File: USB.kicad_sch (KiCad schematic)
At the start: 13 parts, among them J2 USB_B_Micro, U6 FT230XS, U7 USBLC6-2SC6

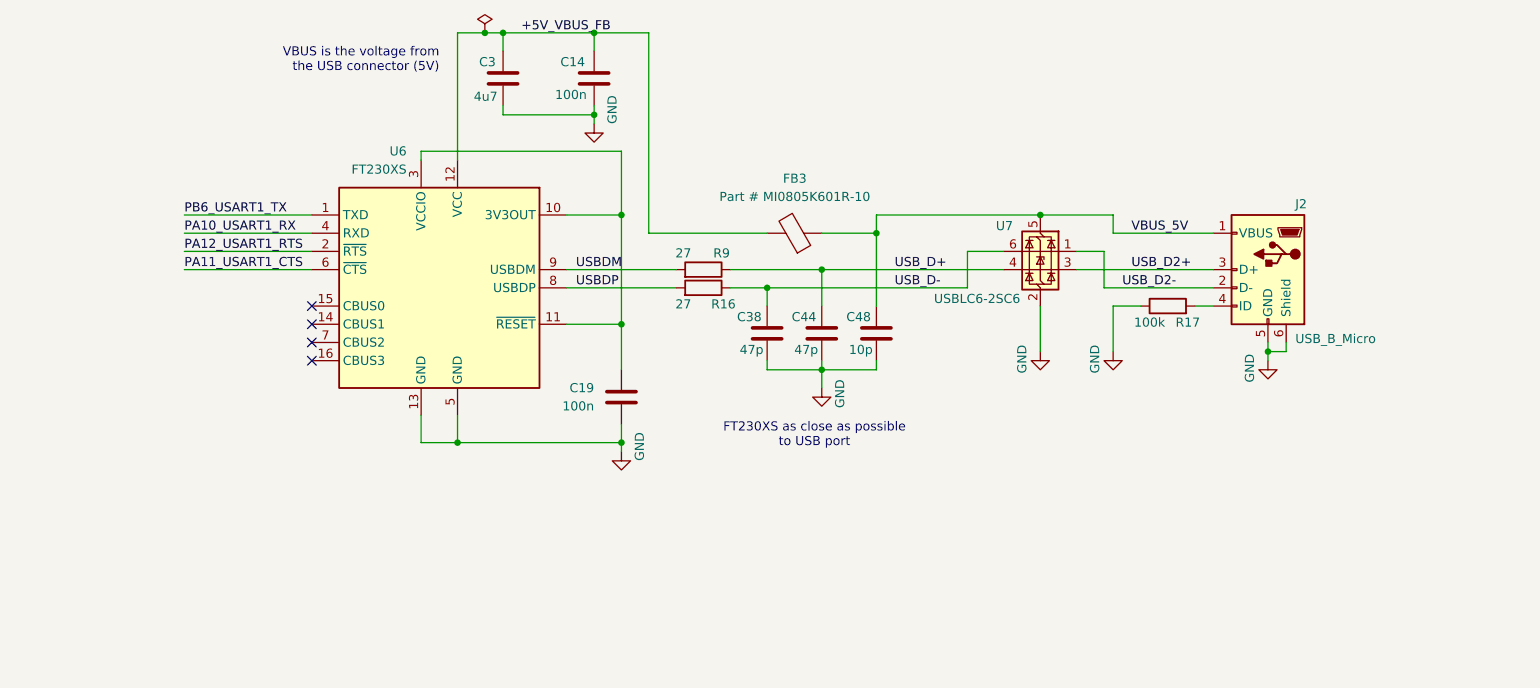
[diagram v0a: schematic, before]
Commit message: Update
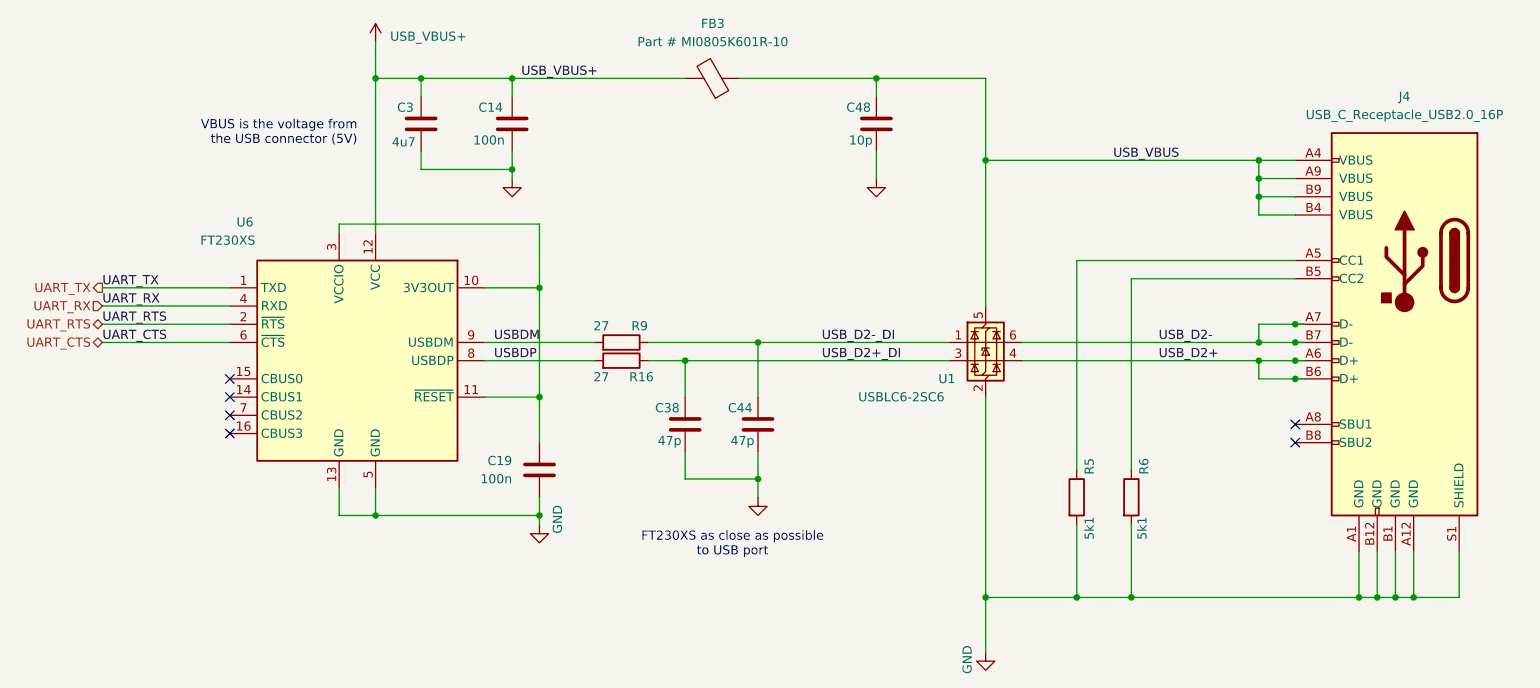
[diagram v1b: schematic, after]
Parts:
- removed J2: USB_B_Micro, Connector_USB:USB_Micro-B_XKB_U254-051T-4BH83-F1S, symbol Connector:USB_B_Micro
- removed R17: 100k, Resistor_SMD:R_0805_2012Metric, symbol Device:R
- removed U7: USBLC6-2SC6, Package_TO_SOT_SMD:SOT-23-6, symbol Power_Protection:USBLC6-2SC6
- added J4: USB_C_Receptacle_USB2.0_16P, Connector_USB:USB_C_Receptacle_HRO_TYPE-C-31-M-12, symbol Connector:USB_C_Receptacle_USB2.0_16P
- added R5, R6: 5k1, Resistor_SMD:R_0805_2012Metric, symbol Device:R
- added U1: USBLC6-2SC6, Package_TO_SOT_SMD:SOT-23-6, symbol Power_Protection:USBLC6-2SC6
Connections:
- net GND: now also J4.A1 (GND), J4.A12 (GND), J4.B1 (GND), J4.B12 (GND), J4.S1 (SHIELD), R5.2, R6.2, U1.2 (GND)
- net USB_D2+: now also J4.A6 (D+), J4.B6 (D+), U1.4 (I/O2)
- net USB_D2-: now also J4.A7 (D-), J4.B7 (D-), U1.6 (I/O1)
- net +5V_VBUS_FB renamed USB_VBUS+
- net PA10_USART1_RX renamed UART_RX
- net PA11_USART1_CTS renamed UART_CTS
- net PA12_USART1_RTS renamed UART_RTS
- net PB6_USART1_TX renamed UART_TX
- net USB_D+ renamed USB_D2-_DI
- net USB_D2-_DI: now also U1.1 (I/O1)
- net USB_D- renamed USB_D2+_DI
- net USB_D2+_DI: now also U1.3 (I/O2)
- net VBUS_5V renamed USB_VBUS
- net USB_VBUS: now also J4.A4 (VBUS), J4.A9 (VBUS), J4.B4 (VBUS), J4.B9 (VBUS), U1.5 (VBUS)
- new net: J4.B5 (CC2), R6.1
- new net: J4.A5 (CC1), R5.1
- no-connect marks 4 -> 6
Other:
- moved on the sheet: C14, C19, C3, C38, C44, C48, FB3, R16, R9, U6
